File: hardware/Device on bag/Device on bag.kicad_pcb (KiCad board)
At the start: 2 copper layers, 62.2 x 53.3 mm, 5 parts, among them SW1 SW_DIP_x01, U1 STEVAL-MKI215V1, U2 D1_mini_battery_shield, U3 ESP32-DEVKIT-V1

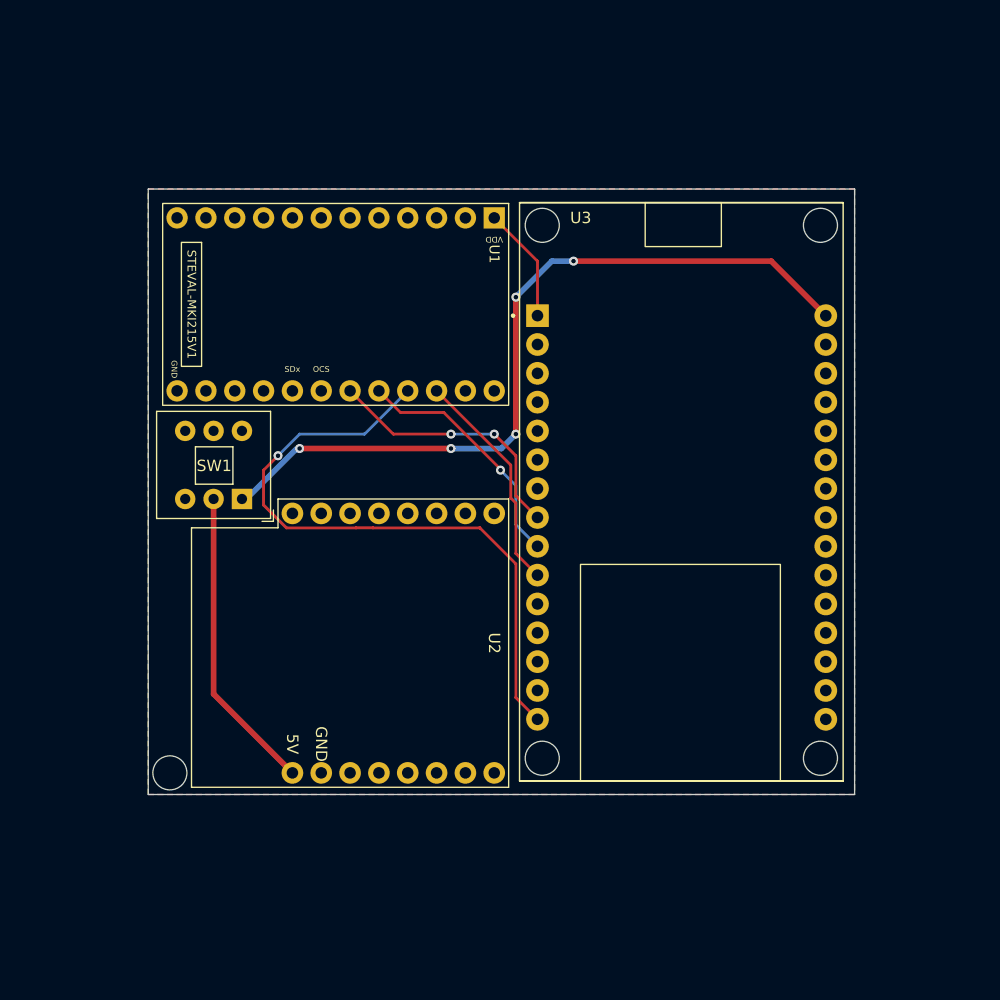
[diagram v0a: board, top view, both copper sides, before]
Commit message: final commit i hope
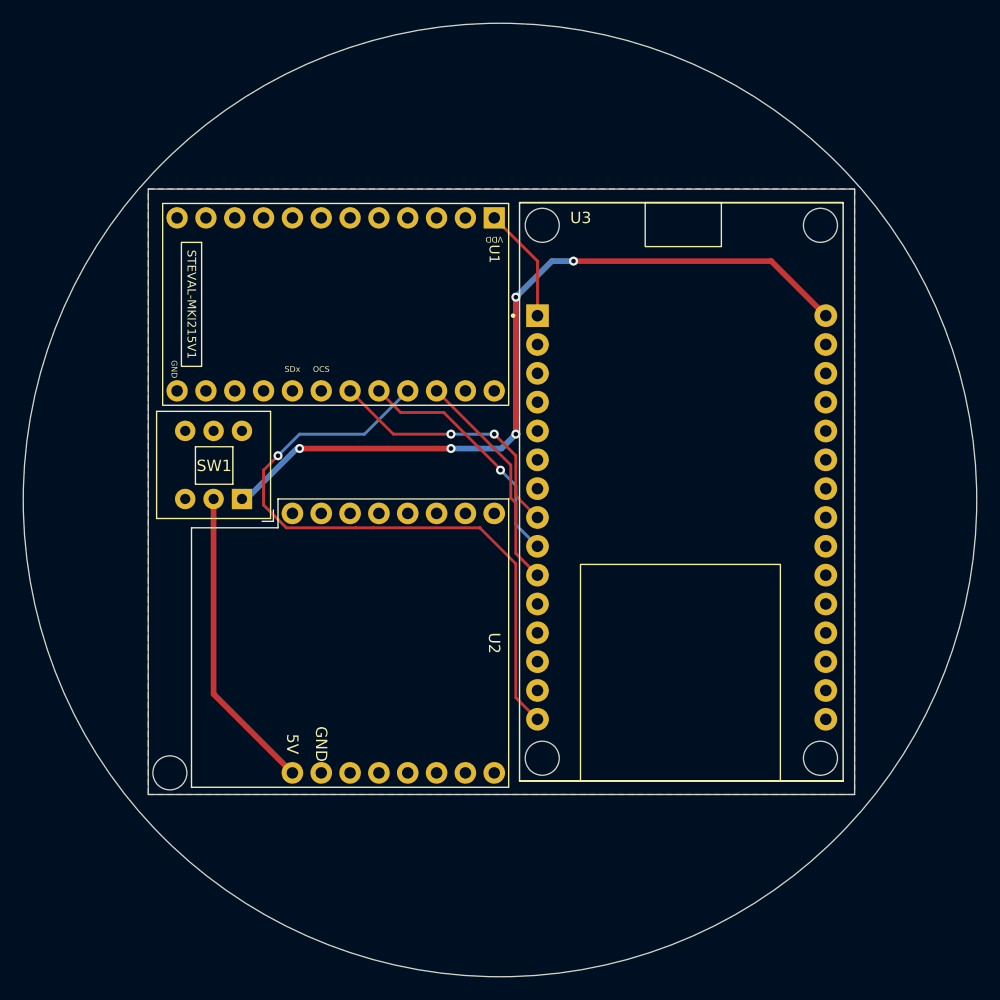
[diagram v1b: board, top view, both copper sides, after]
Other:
- board size 62.2 x 53.3 mm -> 84 x 84 mm

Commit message: init
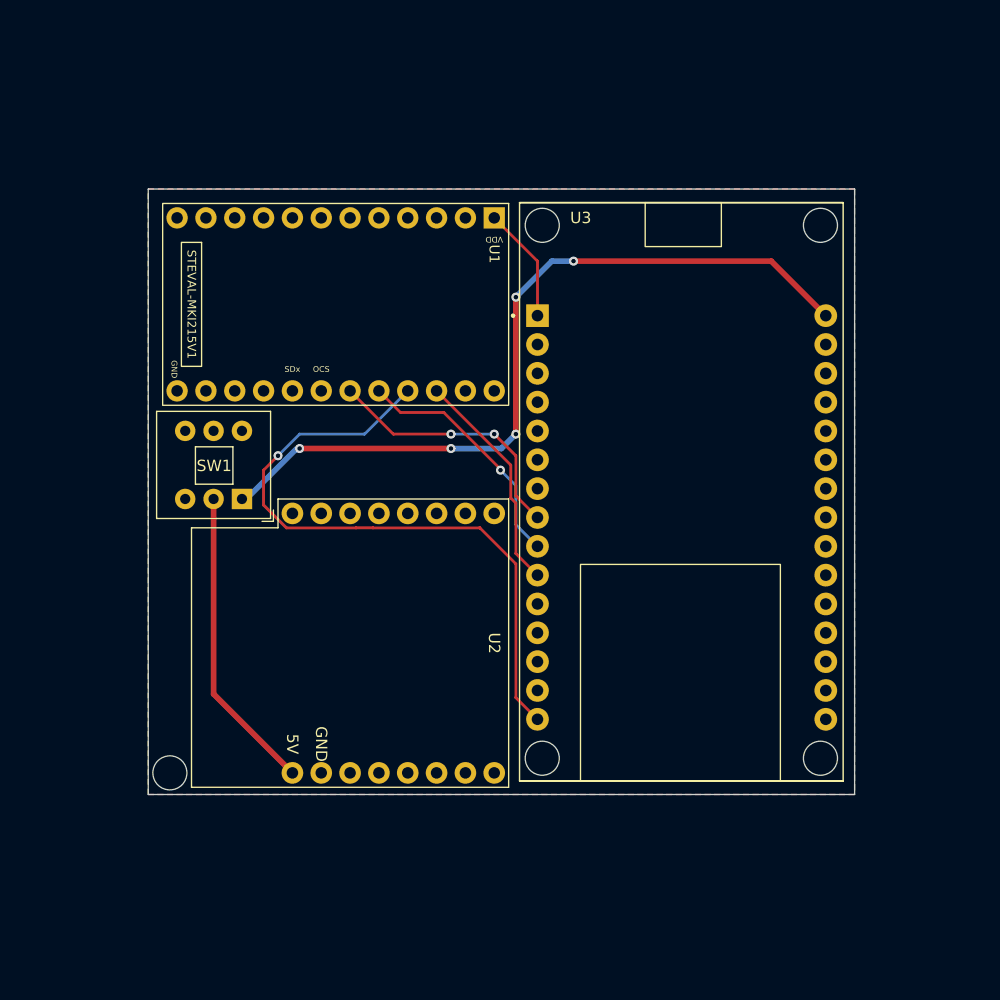
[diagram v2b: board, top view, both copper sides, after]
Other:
- board size 84 x 84 mm -> 62.2 x 53.3 mm
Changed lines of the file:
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@@
     (pad_to_mask_clearance 0)
     (pcbplotparams
-      (layerselection 0x00010fc_ffffffff)
-      (plot_on_all_layers_selection 0x0000000_00000000)
+      (layerselection 0x000103f_ffffffff)
+      (plot_on_all_layers_selection 0x00000cc_80000001)
       (disableapertmacros false)
       (usegerberextensions true)
@@
       (hpglpendiameter 15.000000)
       (dxfpolygonmode true)
-      (dxfimperialunits true)
+      (dxfimperialunits false)
       (dxfusepcbnewfont true)
       (psnegative false)
@@
       (sketchpadsonfab false)
       (subtractmaskfromsilk true)
-      (outputformat 1)
+      (outputformat 3)
       (mirror false)
       (drillshape 0)
       (scaleselection 1)
-      (outputdirectory "")
+      (outputdirectory "../Assembly/")
     )
   )
@@
   (gr_rect (start 105.41 52.705) (end 167.64 106.045)
     (stroke (width 0.1) (type solid)) (fill none) (layer "Edge.Cuts"))
-  (gr_circle (center 136.398 80.1) (end 178.398 80.1)
-    (stroke (width 0.1) (type default)) (fill none) (layer "Edge.Cuts"))
   (dimension (type aligned) (layer "Edge.Cuts")
     (pts (xy 167.64 52.705) (xy 167.64 106.045))
